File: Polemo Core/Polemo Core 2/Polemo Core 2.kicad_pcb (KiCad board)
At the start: 4 copper layers, 40 x 100 mm, 174 parts, among them P1 Header-Male-2.54_2x2, P2 Header-Male-2.54_2x2, Q1 BC847_C2910145, Q2 MMBT5551LT1G, Q3 AO3401A, Q4 AO3401A, Q5 MMBT5551LT1G, U1 ATSAML21G18B-AUT, U10 74LVC1G08GV,125, U11 LT3014BHVES5#TRMPBF, U12 TXU0202DCUR, U13 TLV7031DBVR, U14 TLR341G-GTR, U15 803-87-006-10-001101, U2 XC6209F332MR-G, U3 MC14043BDR2G, U4 LMV793MFX/NOPB, U5 TPS7A2030PDBVR, U6 TLV3201AIDBVT, U7 OPA357AIDBVR, U8 TLR341G-GTR, U9 MF-ASML020/6-2, X1 32.768kHz

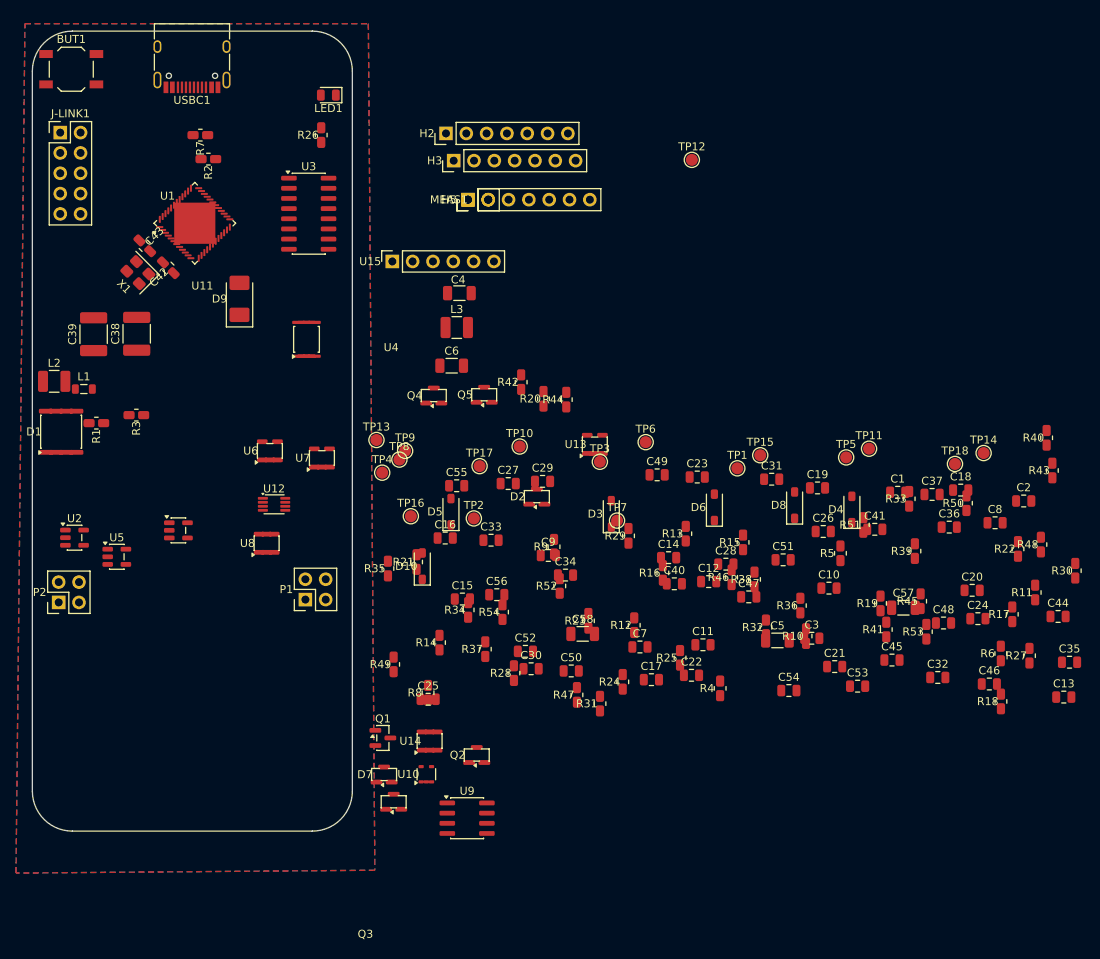
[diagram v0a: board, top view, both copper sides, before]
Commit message: Added README.md and update many files
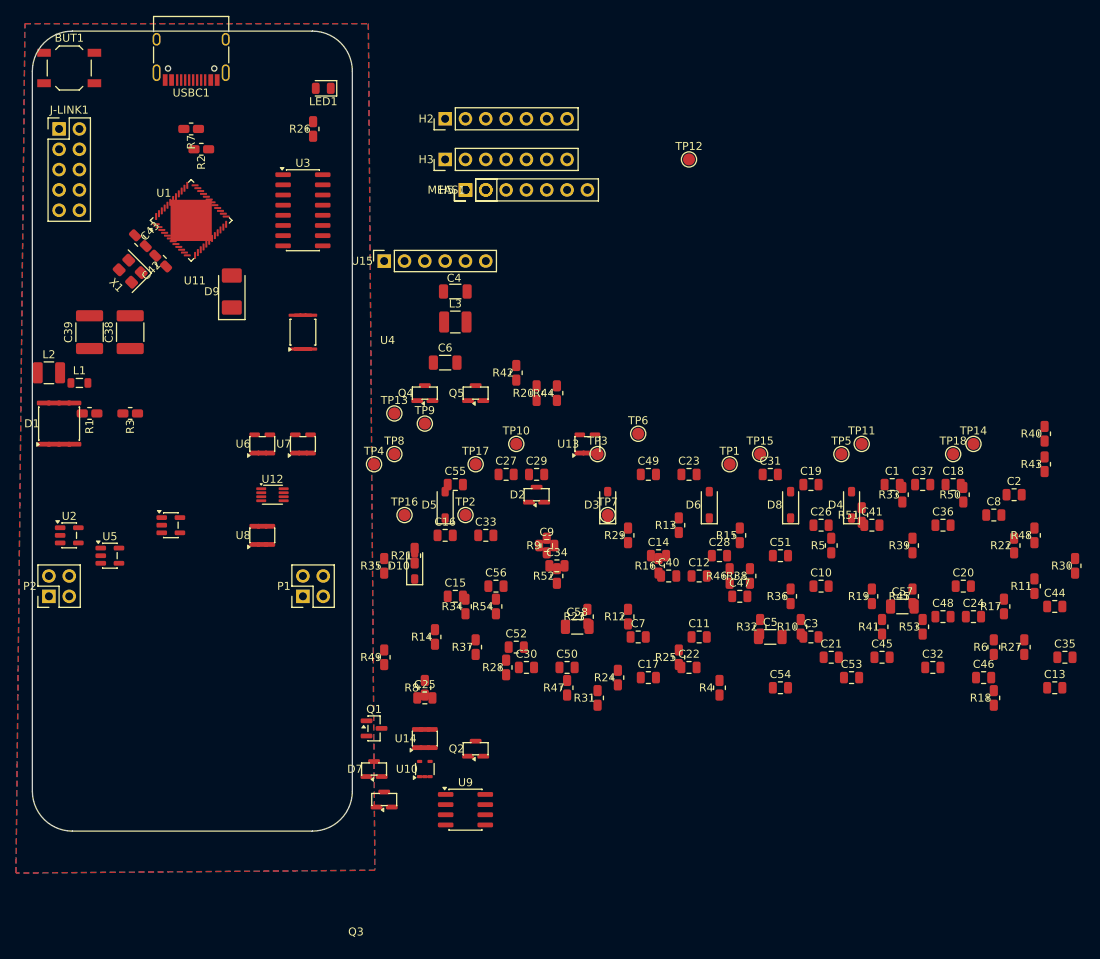
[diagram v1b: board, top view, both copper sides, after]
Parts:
- moved TP9 4.21 mm to (99.1, 99.1)
- moved TP13 4.00 mm to (95.2, 97.8)
- moved U7 2.95 mm to (83.8, 101.6)
- moved H2 1.83 mm to (101.6, 61.0)
- moved TP14 1.71 mm to (167.6, 101.6)
- moved C37 1.71 mm to (161.3, 106.7)
- moved R36 1.68 mm to (144.8, 120.7)
- moved Q1 1.63 mm to (92.7, 137.2)
- moved C13 1.62 mm to (177.8, 132.1)
- moved C34 1.58 mm to (115.6, 116.8)
- moved R47 1.52 mm to (116.8, 132.1)
- moved R2 1.51 mm to (71.1, 64.8)
- moved R5 1.50 mm to (149.9, 114.3)
- moved R49 1.48 mm to (94.0, 128.3)
- moved R1 1.48 mm to (57.1, 97.8)
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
